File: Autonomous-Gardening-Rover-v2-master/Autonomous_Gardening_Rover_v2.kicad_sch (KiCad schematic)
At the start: 64 parts, among them J1 12V BATTERY POWER, J10 SENSORS, J15 Conn_01x02_Pin, J2 USB_B_Micro, J7 MPU SIGNAL, J9 MPU POWER, Q1 BC107, Q2 BC107, Q3 AO4485, SW1 SW_Push, SW2 SW_Push, U1 ESP32-S3-WROOM-1, U2 CP2104, U6 MPU-6500, U7 TPS62933DRLR

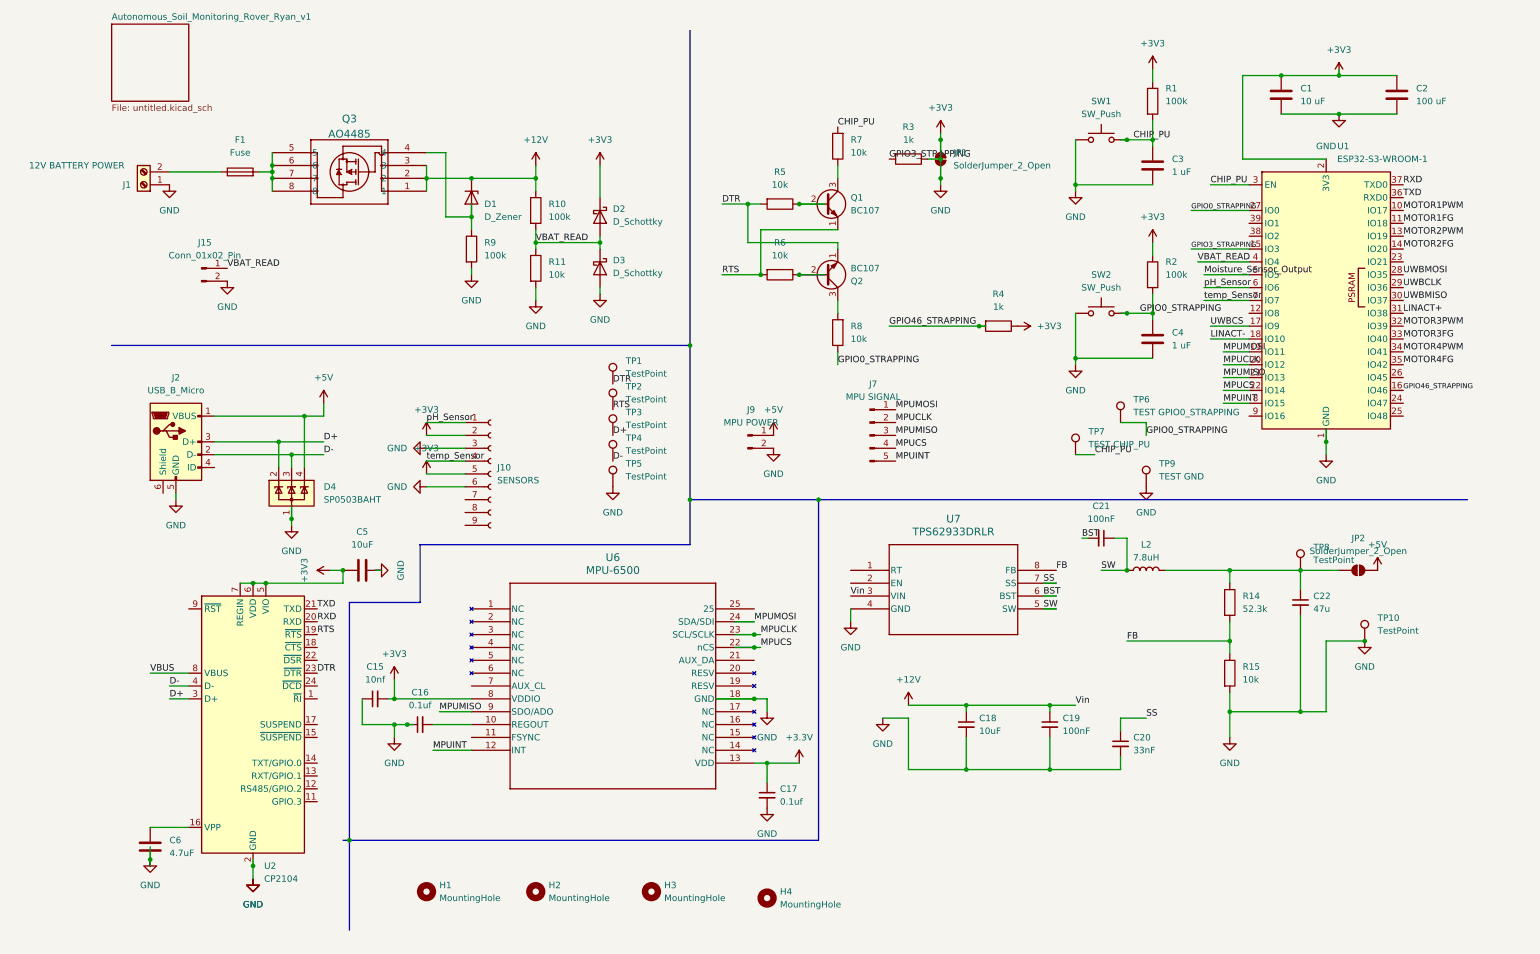
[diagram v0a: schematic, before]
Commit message: Update PCB
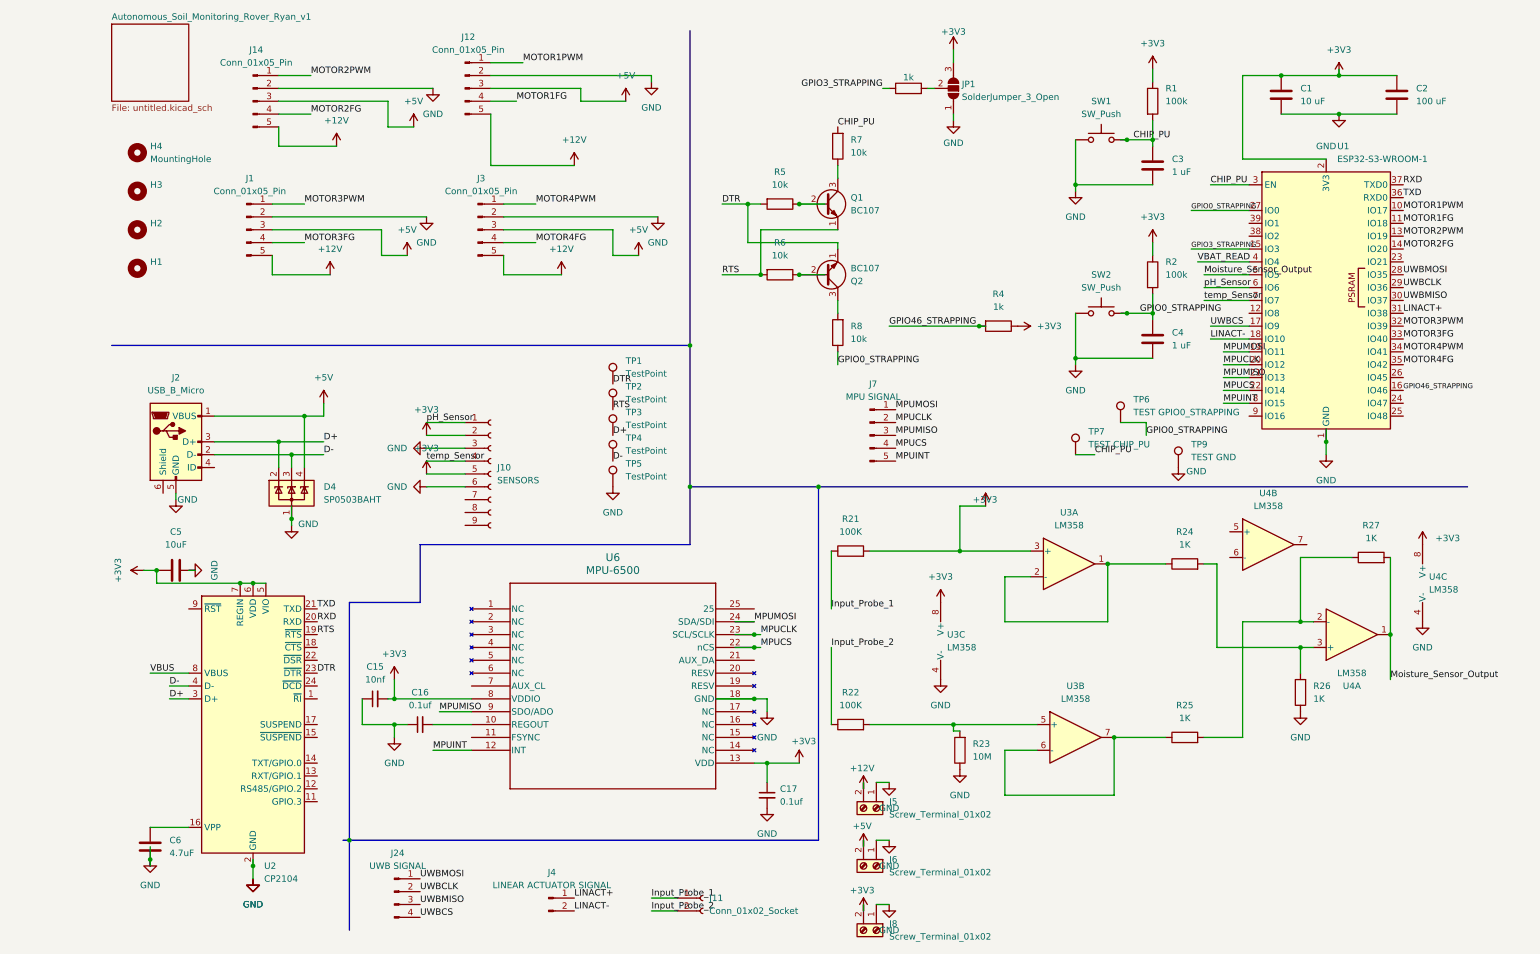
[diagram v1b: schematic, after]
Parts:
- removed C18: 10uF, Capacitor_SMD:C_0805_2012Metric_Pad1.18x1.45mm_HandSolder, symbol Device:C_Small
- removed C19, C21: 100nF, Capacitor_SMD:C_0805_2012Metric_Pad1.18x1.45mm_HandSolder, symbol Device:C_Small
- removed C20: 33nF, Capacitor_SMD:C_0805_2012Metric_Pad1.18x1.45mm_HandSolder, symbol Device:C_Small
- removed C22: 47u, Capacitor_SMD:C_0805_2012Metric_Pad1.18x1.45mm_HandSolder, symbol Device:C_Small
- removed D1: D_Zener, Diode_SMD:D_SOD-123, symbol Device:D_Zener
- removed D2, D3: D_Schottky, Package_TO_SOT_SMD:TSOT-23_HandSoldering, symbol Device:D_Schottky
- removed F1: Fuse, Fuse:Fuseholder_Littelfuse_Nano2_154x, symbol Device:Fuse
- removed J1: 12V BATTERY POWER, TerminalBlock_Phoenix:TerminalBlock_Phoenix_MKDS-1,5-2-5.08_1x02_P5.08mm_Horizontal, symbol Connector:Screw_Terminal_01x02
- removed J15: Conn_01x02_Pin, TerminalBlock_Phoenix:TerminalBlock_Phoenix_MKDS-1,5-2-5.08_1x02_P5.08mm_Horizontal, symbol Connector:Conn_01x02_Pin
- removed J9: MPU POWER, TerminalBlock_Phoenix:TerminalBlock_Phoenix_MKDS-1,5-2-5.08_1x02_P5.08mm_Horizontal, symbol Connector:Conn_01x02_Pin
- removed JP1, JP2: SolderJumper_2_Open, Jumper:SolderJumper-2_P1.3mm_Open_RoundedPad1.0x1.5mm, symbol Jumper:SolderJumper_2_Open
- removed L2: 7.8uH, Inductor_Custom:Inductor_Custom, symbol Device:L
- removed Q3: AO4485, AO4485:SO8SOP-8L_AOS, symbol local_symbols:AO4485
- removed R10, R9: 100k, Resistor_SMD:R_0805_2012Metric_Pad1.20x1.40mm_HandSolder, symbol Device:R
- removed R11, R15: 10k, Resistor_SMD:R_0805_2012Metric_Pad1.20x1.40mm_HandSolder, symbol Device:R
- removed R14: 52.3k, Resistor_SMD:R_0805_2012Metric_Pad1.20x1.40mm_HandSolder, symbol Device:R
- removed R3: 1k, Resistor_SMD:R_0805_2012Metric_Pad1.20x1.40mm_HandSolder, symbol Device:R
- removed TP10, TP8: TestPoint, TestPoint:TestPoint_Pad_2.5x2.5mm, symbol Connector:TestPoint
- removed U7: TPS62933DRLR, TSP62933DRLR:SOT-5X3-8_DRL_TEX, symbol TPS62933DRLR:TPS62933DRLR
- added J1, J12, J14, J3: Conn_01x05_Pin, TerminalBlock_Phoenix:TerminalBlock_Phoenix_MKDS-1,5-5-5.08_1x05_P5.08mm_Horizontal, symbol Connector:Conn_01x05_Pin
- added J11: Conn_01x02_Socket, TerminalBlock_Phoenix:TerminalBlock_Phoenix_MKDS-1,5-2-5.08_1x02_P5.08mm_Horizontal, symbol Connector:Conn_01x02_Socket
- added J24: UWB SIGNAL, TerminalBlock_Phoenix:TerminalBlock_Phoenix_MKDS-1,5-4-5.08_1x04_P5.08mm_Horizontal, symbol Connector:Conn_01x04_Pin
- added J4: LINEAR ACTUATOR SIGNAL, TerminalBlock_Phoenix:TerminalBlock_Phoenix_MKDS-1,5-2-5.08_1x02_P5.08mm_Horizontal, symbol Connector:Conn_01x02_Pin
- added J5, J6, J8: Screw_Terminal_01x02, TerminalBlock_Phoenix:TerminalBlock_Phoenix_MKDS-1,5-2-5.08_1x02_P5.08mm_Horizontal, symbol Connector:Screw_Terminal_01x02
- added JP1: SolderJumper_3_Open, Jumper:SolderJumper-3_P2.0mm_Open_TrianglePad1.0x1.5mm, symbol Jumper:SolderJumper_3_Open
- added R21, R22: 100K, Resistor_SMD:R_0805_2012Metric_Pad1.20x1.40mm_HandSolder, symbol Device:R
- added R23: 10M, Resistor_SMD:R_0805_2012Metric_Pad1.20x1.40mm_HandSolder, symbol Device:R
- added R24, R25, R26, R27: 1K, Resistor_SMD:R_0805_2012Metric_Pad1.20x1.40mm_HandSolder, symbol Device:R
- added R3: 1k, Resistor_SMD:R_0805_2012Metric, symbol basic:R
- added U3, U4: LM358, LM358P:P8, symbol Amplifier_Operational:LM358
- SW1, SW2: footprint Button_Switch_SMD:SW_DIP_SPSTx01_Slide_Copal_CHS-01A_W5.08mm_P1.27mm_JPin -> Button_Switch_THT:SW_PUSH_6mm_H5mm
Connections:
- net +3.3V is gone; now on net +3V3: C17.1, U6.13 (VDD)
- net +12V: now also J1.5 (Pin_5), J12.5 (Pin_5), J14.5 (Pin_5), J3.5 (Pin_5), J5.2 (Pin_2)
- net +3V3: now also J8.2 (Pin_2), JP1.3 (B), R21.2, U3.3 (+), U3.8 (V+), U4.8 (V+); no longer C1.2, C15.1, C16.1, C17.2, C2.2, C3.2, C4.2, C5.2, C6.2, D4.1 (A), J10.3 (Pin_3), J10.6 (Pin_6), J2.5 (GND), SW1.1, SW2.1, TP5.1, TP9.1, U1.1 (GND), U1.40 (GND), U1.41 (GND), U2.2 (GND), U2.25 (GND), U6.18 (GND)
- net +5V: now also J1.3 (Pin_3), J12.3 (Pin_3), J14.3 (Pin_3), J3.3 (Pin_3), J6.2 (Pin_2)
- net GPIO3_STRAPPING: now also R3.1
- net LINACT+: now also J4.1 (Pin_1)
- net LINACT-: now also J4.2 (Pin_2)
- net MOTOR1FG: now also J12.4 (Pin_4)
- net MOTOR1PWM: now also J12.1 (Pin_1)
- net MOTOR2FG: now also J14.4 (Pin_4)
- net MOTOR2PWM: now also J14.1 (Pin_1)
- net MOTOR3FG: now also J1.4 (Pin_4)
- net MOTOR3PWM: now also J1.1 (Pin_1)
- net MOTOR4FG: now also J3.4 (Pin_4)
- net MOTOR4PWM: now also J3.1 (Pin_1)
- net Moisture_Sensor_Output: now also R27.2, U4.1
- net UWBCLK: now also J24.2 (Pin_2)
- net UWBCS: now also J24.4 (Pin_4)
- net UWBMISO: now also J24.3 (Pin_3)
- net UWBMOSI: now also J24.1 (Pin_1)
- new net: R25.2, R27.1, U4.2 (-)
- new net: R24.2, R26.2, U4.3 (+)
- new net: R22.2, R23.2, U3.5 (+)
- new net: R25.1, U3.6 (-), U3.7
- new net: R24.1, U3.1, U3.2 (-)
- new net: JP1.2 (C), R3.2
- new net GND: C1.2, C15.1, C16.1, C17.2, C2.2, C3.2, C4.2, C5.2, C6.2, D4.1 (A), J1.2 (Pin_2), J10.3 (Pin_3), J10.6 (Pin_6), J12.2 (Pin_2), J14.2 (Pin_2), J2.5 (GND), J3.2 (Pin_2), J5.1 (Pin_1), J6.1 (Pin_1), J8.1 (Pin_1), JP1.1 (A), R23.1, R26.1, SW1.1, SW2.1, TP5.1, TP9.1, U1.1 (GND), U1.40 (GND), U1.41 (GND), U2.2 (GND), U2.25 (GND), U3.4 (V-), U4.4 (V-), U6.18 (GND)
- new net Input_Probe_1: J11.1 (Pin_1), R21.1
- new net Input_Probe_2: J11.2 (Pin_2), R22.1
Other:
- moved on the sheet: C5, H1, H2, H3, H4, TP9
